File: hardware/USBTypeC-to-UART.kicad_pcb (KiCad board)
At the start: 2 copper layers, 28.2 x 17.5 mm, 5 parts, among them J1 USB-C, J2 Header, U1 CP2102N

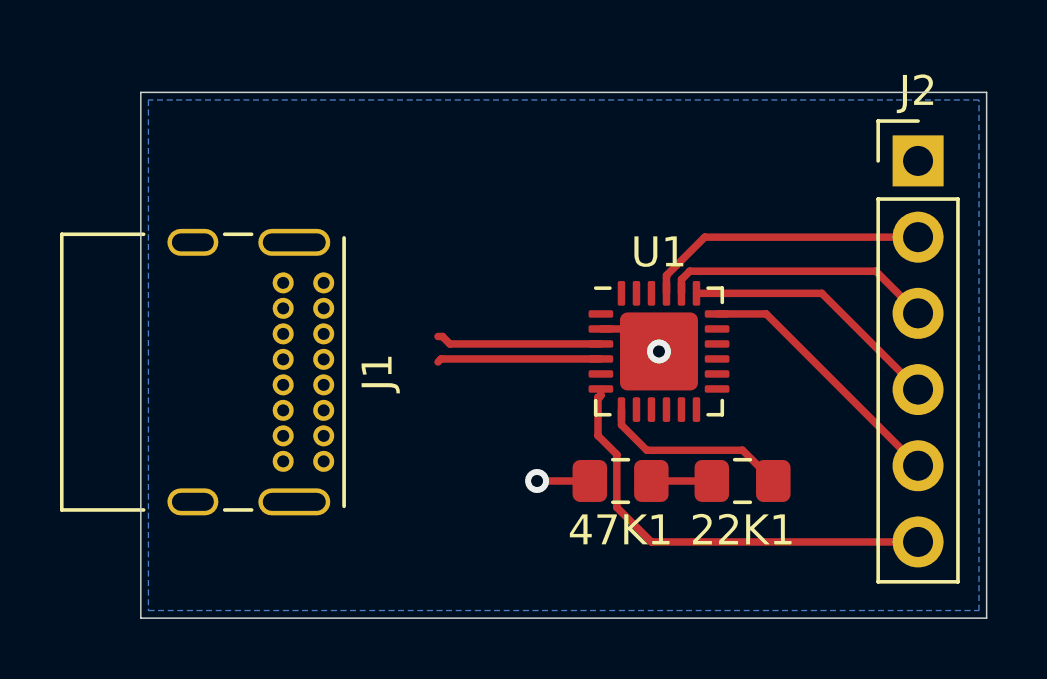
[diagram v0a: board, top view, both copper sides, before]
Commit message: layout
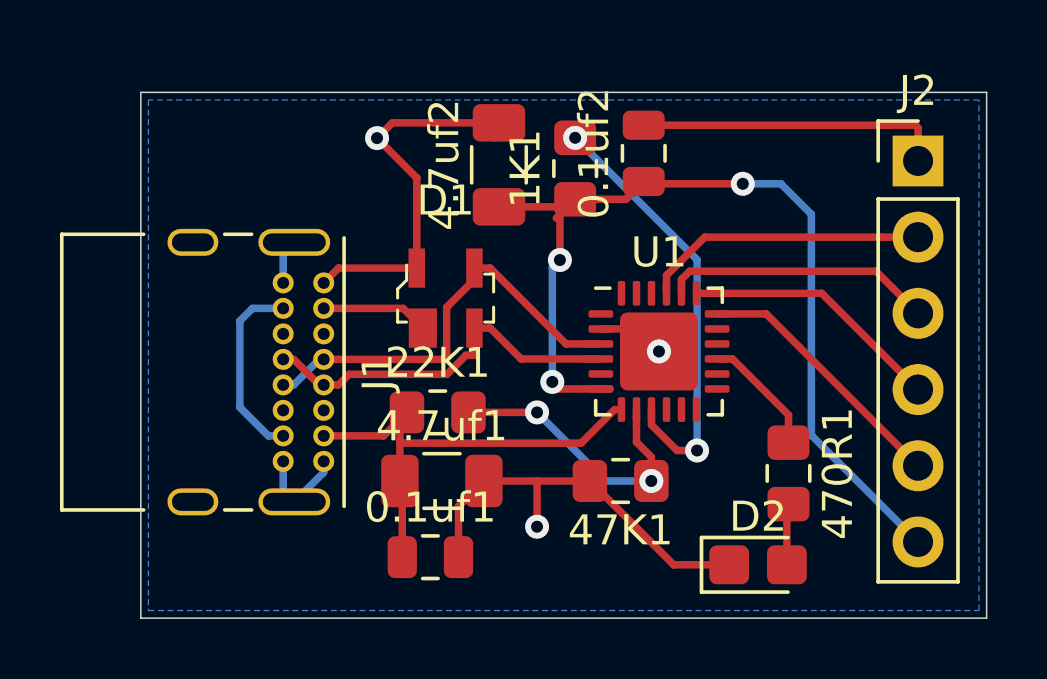
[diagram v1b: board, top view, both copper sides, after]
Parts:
- added 0.1uf1: C, Capacitor_SMD:C_0805_2012Metric, F.Cu at (118.9, 124.7)
- added 0.1uf2: C, Capacitor_SMD:C_0805_2012Metric, F.Cu at (126.0, 111.3)
- added 1K1: R, Resistor_SMD:R_0805_2012Metric_Pad1.15x1.40mm_HandSolder, F.Cu at (123.7, 111.8)
- added 4.7uf1: C, Capacitor_SMD:C_1206_3216Metric, F.Cu at (119.3, 122.2)
- added 4.7uf2: C, Capacitor_SMD:C_1206_3216Metric, F.Cu at (121.2, 111.6)
- added 470R1: R, Resistor_SMD:R_0805_2012Metric_Pad1.15x1.40mm_HandSolder, F.Cu at (130.8, 121.9)
- added D1: SP0503BAHTG, digikey-footprints:SOT-143-4, F.Cu at (119.4, 116.1)
- added D2: LED, LED_SMD:LED_0805_2012Metric_Castellated, F.Cu at (129.8, 125.0)
- J1: value USB-C -> USB_C
- U1: value CP2102N -> CP2102N-A01-GQFN24
- moved 22K1 10.4 mm to (119.1, 119.9), turned to 0 degrees
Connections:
- U1 pad 15: (no net) -> /SUSPENDn
- U1 pad 9: (no net) -> Net-(1K1-Pad2)
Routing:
- net GND: track 4.01 -> 43.7 mm, vias 2 -> 3
- net /VBUS: track 6.35 -> 25.8 mm
- net VDD: track 14.8 -> 32.9 mm, vias 0 -> 3
- net Net-(1K1-Pad2): track 0.00 -> 14.5 mm, vias 0 -> 2
- net /D+: track 5.53 -> 14.4 mm
- net Net-(22K1-Pad2): track 2.01 -> 9.63 mm, vias 0 -> 2
- net /D-: track 5.47 -> 12.7 mm
- net /SUSPENDn: track 0.00 -> 4.08 mm
- net Net-(470R1-Pad2): track 0.00 -> 2.05 mm
